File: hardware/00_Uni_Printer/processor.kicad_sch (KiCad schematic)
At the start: 23 parts, among them IC2 MT25QL256ABA1EW7-0SIT_TR, U1 STM32H743VIT6, Y1 ABM7-25.000MHZ-D2Y-T

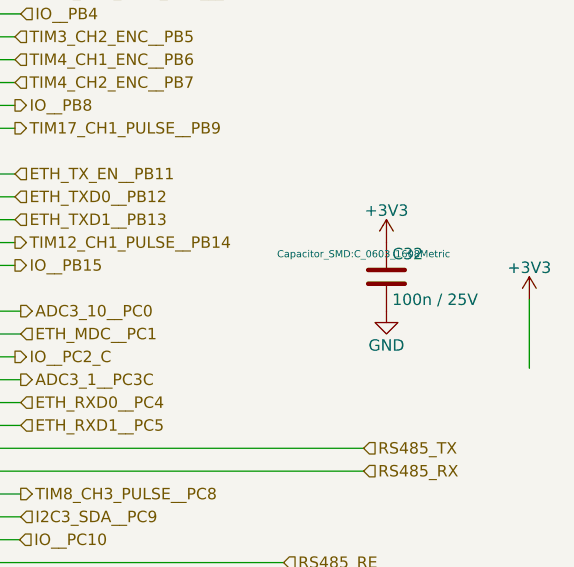
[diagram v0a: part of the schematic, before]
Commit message: Fixes in PCB design
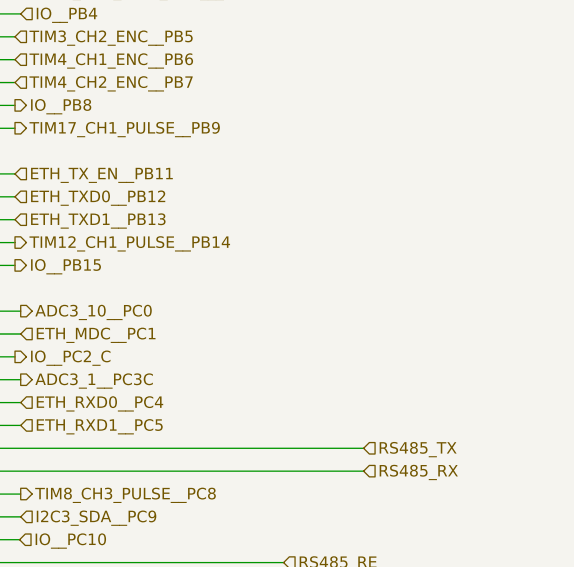
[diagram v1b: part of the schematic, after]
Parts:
- removed C32: 100n / 25V, Capacitor_SMD:C_0603_1608Metric, symbol mfc_base_lib:C
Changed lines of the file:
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@@
-    (stroke (width 0) (type solid) (color 0 0 0 0))
-  )
-  (wire (pts (xy 244.475 125.095) (xy 244.475 132.715))
     (stroke (width 0) (type solid) (color 0 0 0 0))
   )
@@
     (pin "1")
   )
-  (symbol (lib_id "mfc_base_lib:+3V3") (at 228.6 118.745 0) (unit 1)
-    (in_bom yes) (on_board yes)
-    (property "Reference" "#PWR0106" (id 0) (at 228.6 122.555 0)
-      (effects (font (size 1.27 1.27)) hide)
-    )
-    (property "Value" "+3V3" (id 1) (at 228.6 115.189 0))
-    (property "Footprint" "" (id 2) (at 228.6 118.745 0)
-      (effects (font (size 1.27 1.27)) hide)
-    )
-    (property "Datasheet" "" (id 3) (at 228.6 118.745 0)
-      (effects (font (size 1.27 1.27)) hide)
-    )
-    (pin "1")
-  )
   (symbol (lib_id "Jumper:Jumper_2_Open") (at 26.035 45.085 90) (unit 1)
     (in_bom yes) (on_board yes) (fields_autoplaced)
@@
     (property "Datasheet" "~" (id 3) (at 26.035 45.085 0)
       (effects (font (size 1.27 1.27)) hide)
-    )
-    (pin "1")
-    (pin "2")
-  )
-  (symbol (lib_id "mfc_base_lib:C") (at 228.6 122.555 0) (unit 1)
-    (in_bom yes) (on_board yes)
-    (property "Reference" "C32" (id 0) (at 229.235 120.015 0)
-      (effects (font (size 1.27 1.27)) (justify left))
-    )
-    (property "Value" "100n / 25V" (id 1) (at 229.235 125.095 0)
-      (effects (font (size 1.27 1.27)) (justify left))
-    )
-    (property "Footprint" "Capacitor_SMD:C_0603_1608Metric" (id 2) (at 226.06 120.015 0)
-      (effects (font (size 0.7874 0.7874)))
-    )
-    (property "Datasheet" "" (id 3) (at 228.6 122.555 0)
-      (effects (font (size 1.27 1.27)) hide)
-    )
-    (property "Category" "Capacitor" (id 4) (at 228.6 122.555 0)
-      (effects (font (size 1.524 1.524)) hide)
     )
     (pin "1")
@@
       (effects (font (size 1.27 1.27)) hide)
     )
-    (pin "1")
-  )
-  (symbol (lib_id "mfc_base_lib:+3V3") (at 244.475 125.095 0) (unit 1)
-    (in_bom yes) (on_board yes)
-    (property "Reference" "#PWR0103" (id 0) (at 244.475 128.905 0)
-      (effects (font (size 1.27 1.27)) hide)
-    )
-    (property "Value" "+3V3" (id 1) (at 244.475 121.539 0))
-    (property "Footprint" "" (id 2) (at 244.475 125.095 0)
-      (effects (font (size 1.27 1.27)) hide)
-    )
-    (property "Datasheet" "" (id 3) (at 244.475 125.095 0)
-      (effects (font (size 1.27 1.27)) hide)
-    )
-    (pin "1")
-  )
-  (symbol (lib_id "mfc_base_lib:GND") (at 228.6 126.365 0) (unit 1)
-    (in_bom yes) (on_board yes)
-    (property "Reference" "#PWR0102" (id 0) (at 228.6 132.715 0)
-      (effects (font (size 1.27 1.27)) hide)
-    )
-    (property "Value" "GND" (id 1) (at 228.6 130.175 0))
-    (property "Footprint" "" (id 2) (at 228.6 126.365 0)
-      (effects (font (size 1.27 1.27)) hide)
-    )
-    (property "Datasheet" "" (id 3) (at 228.6 126.365 0)
-      (effects (font (size 1.27 1.27)) hide)
-    )
